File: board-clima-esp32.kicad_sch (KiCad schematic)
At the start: 54 parts, among them IC1 ESP32-S3-WROOM-1-N4, J1 Conn_01x06_Pin, J2 Screw_Terminal_01x03, J3 Conn_01x04_Pin, J5 Conn_01x05_Pin, J6 USB_C_Receptacle, Q1 AO3400A, Q2 AO3401A, Q3 AO3400A, SW1 RESET, SW2 BOOT, U1 AMS1117-3.3, U3 PC817, U4 PC817

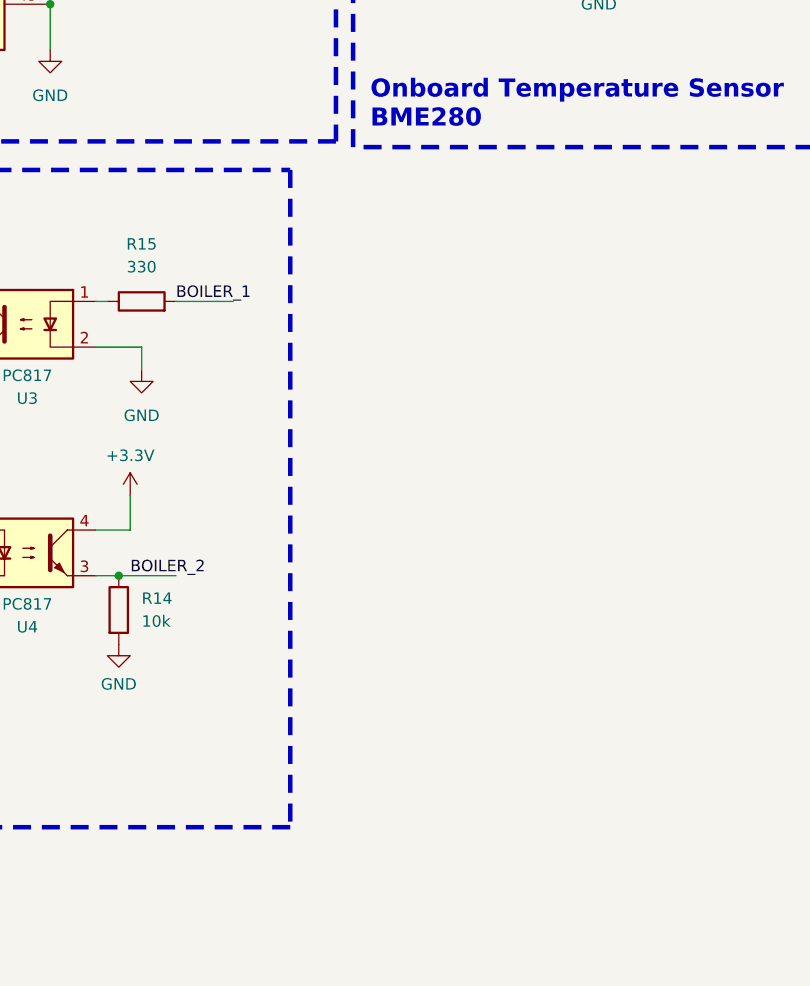
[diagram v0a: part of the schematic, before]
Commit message: drc passes
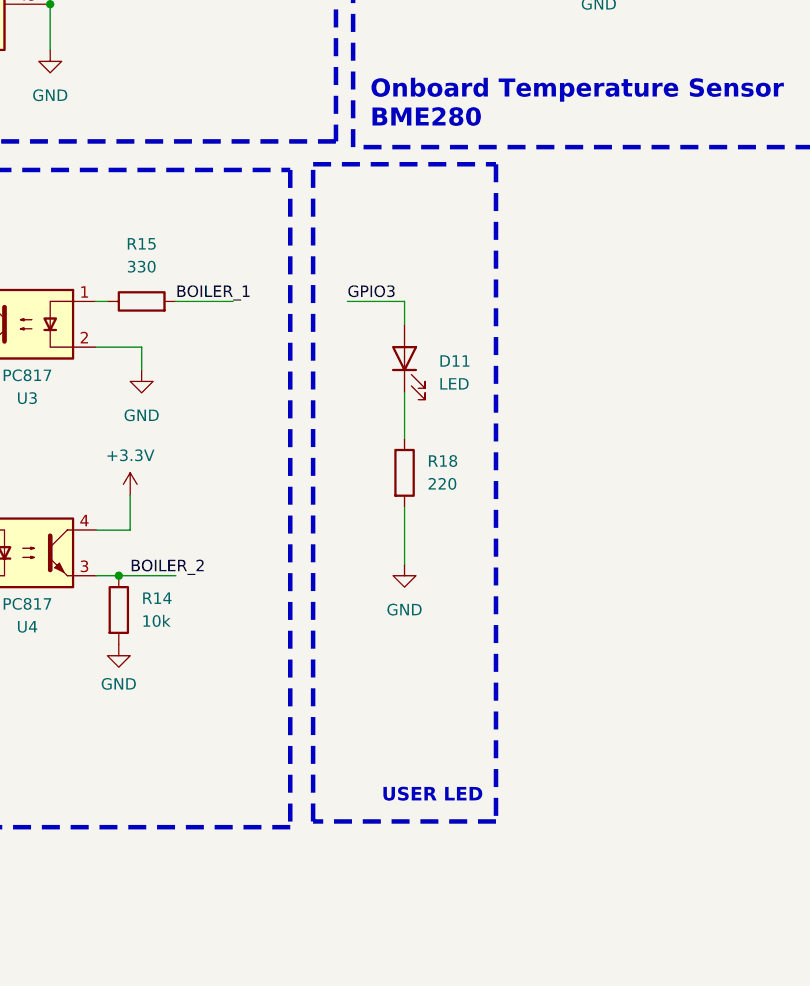
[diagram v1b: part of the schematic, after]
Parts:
- added D11: LED, LED_SMD:LED_0805_2012Metric, symbol Device:LED
- added R18: 220, Resistor_SMD:R_0805_2012Metric, symbol Device:R
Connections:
- net GND: now also R18.2
- net GPIO3: now also D11.2 (A)
- new net: D11.1 (K), R18.1
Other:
- note added: "USER LED"
